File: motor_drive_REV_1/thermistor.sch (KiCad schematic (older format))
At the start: 6 parts, among them J5 Conn_01x02, J6 Conn_01x02

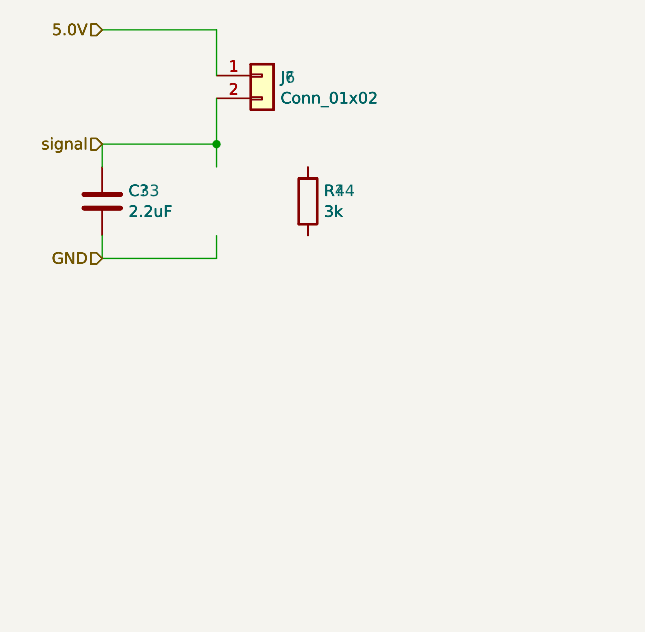
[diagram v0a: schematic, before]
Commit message: started layout
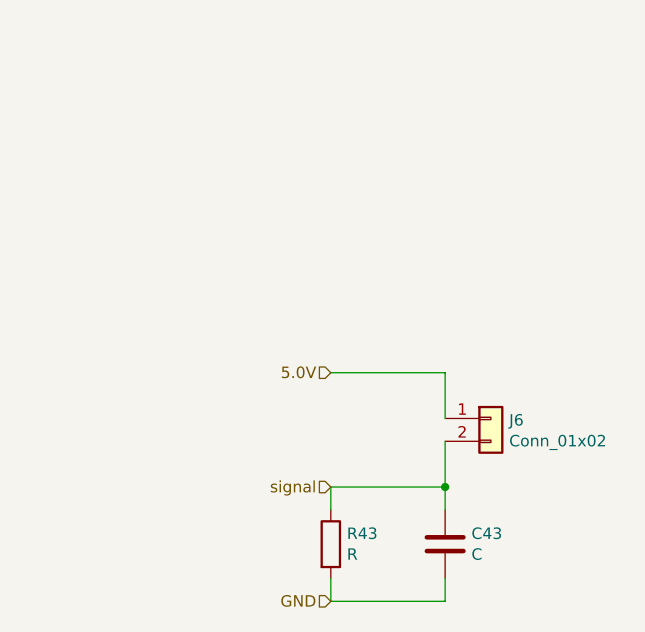
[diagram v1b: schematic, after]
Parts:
- removed C32, C33: 2.2uF, motor_drive_footprints:C_0603_1608Metric, symbol motor_drive:C
- removed J5: Conn_01x02, symbol Connector_Generic:Conn_01x02
- removed R44: 3k, motor_drive_footprints:C_0603_1608Metric, symbol motor_drive:R
- added C43: C, motor_drive_footprints:C_0603_1608Metric, symbol motor_drive:C
- J6: footprint (none) -> motor_drive_footprints:2pos_254
- R43: value 3k -> R
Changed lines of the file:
@@
 $Descr A4 11693 8268
 encoding utf-8
-Sheet 15 15
+Sheet 15 16
 Title ""
 Date ""
@@
 $EndDescr
 $Comp
-L motor_drive:R R44
-U 1 1 5E6227DE
-P 5400 2750
-AR Path="/5E61C379/5E6227DE" Ref="R44"  Part="1"
-AR Path="/5E61FCEC/5E6227DE" Ref="R?"  Part="1"
-AR Path="/5E626DD7/5E6227DE" Ref="R?"  Part="1"
-F 0 "R?" H 5470 2796 50  0000 L CNN
-F 1 "3k" H 5470 2705 50  0000 L CNN
-F 2 "motor_drive_footprints:C_0603_1608Metric" V 5330 2750 50  0001 C CNN
-F 3 "~" H 5400 2750 50  0001 C CNN
-	1    5400 2750
+L motor_drive:R R43
+U 1 1 5E41A8AA
+P 5500 4250
+F 0 "R43" H 5570 4296 50  0000 L CNN
+F 1 "R" H 5570 4205 50  0000 L CNN
+F 2 "motor_drive_footprints:C_0603_1608Metric" V 5430 4250 50  0001 C CNN
+F 3 "~" H 5500 4250 50  0001 C CNN
+	1    5500 4250
 	1    0    0    -1
 $EndComp
 $Comp
-L motor_drive:C C33
-U 1 1 5E6227DF
-P 4500 2750
-AR Path="/5E61C379/5E6227DF" Ref="C33"  Part="1"
-AR Path="/5E61FCEC/5E6227DF" Ref="C?"  Part="1"
-AR Path="/5E626DD7/5E6227DF" Ref="C?"  Part="1"
-F 0 "C?" H 4615 2796 50  0000 L CNN
-F 1 "2.2uF" H 4615 2705 50  0000 L CNN
-F 2 "motor_drive_footprints:C_0603_1608Metric" H 4538 2600 50  0001 C CNN
-F 3 "~" H 4500 2750 50  0001 C CNN
-	1    4500 2750
+L motor_drive:C C43
+U 1 1 5E41AB44
+P 6000 4250
+F 0 "C43" H 6115 4296 50  0000 L CNN
+F 1 "C" H 6115 4205 50  0000 L CNN
+F 2 "motor_drive_footprints:C_0603_1608Metric" H 6038 4100 50  0001 C CNN
+F 3 "~" H 6000 4250 50  0001 C CNN
+	1    6000 4250
 	1    0    0    -1
 $EndComp
 $Comp
 L Connector_Generic:Conn_01x02 J6
-U 1 1 5E6227E0
-P 5200 2200
-AR Path="/5E61C379/5E6227E0" Ref="J6"  Part="1"
-AR Path="/5E61FCEC/5E6227E0" Ref="J?"  Part="1"
-AR Path="/5E626DD7/5E6227E0" Ref="J?"  Part="1"
-F 0 "J?" H 5280 2192 50  0000 L CNN
-F 1 "Conn_01x02" H 5280 2101 50  0000 L CNN
-F 2 "" H 5200 2200 50  0001 C CNN
-F 3 "~" H 5200 2200 50  0001 C CNN
-	1    5200 2200
+U 1 1 5E41B07F
+P 6200 3700
+F 0 "J6" H 6280 3692 50  0000 L CNN
+F 1 "Conn_01x02" H 6280 3601 50  0000 L CNN
+F 2 "motor_drive_footprints:2pos_254" H 6200 3700 50  0001 C CNN
+F 3 "~" H 6200 3700 50  0001 C CNN
+	1    6200 3700
 	1    0    0    -1
 $EndComp
 Wire Wire Line
-	4500 2600 4500 2500
+	5500 3500 6000 3500
 Wire Wire Line
-	4500 2500 5000 2500
+	6000 3500 6000 3700
 Wire Wire Line
-	5000 2500 5000 2600
+	6000 3800 6000 4000
 Wire Wire Line
-	4500 2900 4500 3000
+	5500 4100 5500 4000
 Wire Wire Line
-	4500 3000 5000 3000
+	5500 4000 6000 4000
+Connection ~ 6000 4000
 Wire Wire Line
-	5000 3000 5000 2900
-Text HLabel 4500 3000 0    50   Input ~ 0
+	6000 4000 6000 4100
+Wire Wire Line
+	5500 4400 5500 4500
+Wire Wire Line
+	5500 4500 6000 4500
+Wire Wire Line
+	6000 4500 6000 4400
+Text HLabel 5500 3500 0    50   Input ~ 0
+5.0V
+Text HLabel 5500 4000 0    50   Input ~ 0
+signal
+Text HLabel 5500 4500 0    50   Input ~ 0
 GND
-Text HLabel 4500 2500 0    50   Input ~ 0
-signal
-Text HLabel 4500 2000 0    50   Input ~ 0
-5.0V
-Wire Wire Line
-	4500 2000 5000 2000
-Wire Wire Line
-	5000 2000 5000 2200
-Wire Wire Line
-	5000 2300 5000 2500
-Connection ~ 5000 2500
-$Comp
-L motor_drive:R R?
-U 1 1 5E61C762
-P 5400 2750
-AR Path="/5E61FCEC/5E61C762" Ref="R?"  Part="1"
-AR Path="/5E61C379/5E61C762" Ref="R43"  Part="1"
-AR Path="/5E626DD7/5E61C762" Ref="R?"  Part="1"
-F 0 "R?" H 5470 2796 50  0000 L CNN
-F 1 "3k" H 5470 2705 50  0000 L CNN
-F 2 "motor_drive_footprints:C_0603_1608Metric" V 5330 2750 50  0001 C CNN
-F 3 "~" H 5400 2750 50  0001 C CNN
-	1    5400 2750
-	1    0    0    -1
-$EndComp
-$Comp
-L motor_drive:C C?
-U 1 1 5E61CC30
-P 4500 2750
-AR Path="/5E61FCEC/5E61CC30" Ref="C?"  Part="1"
-AR Path="/5E61C379/5E61CC30" Ref="C32"  Part="1"
-AR Path="/5E626DD7/5E61CC30" Ref="C?"  Part="1"
-F 0 "C?" H 4615 2796 50  0000 L CNN
-F 1 "2.2uF" H 4615 2705 50  0000 L CNN
-F 2 "motor_drive_footprints:C_0603_1608Metric" H 4538 2600 50  0001 C CNN
-F 3 "~" H 4500 2750 50  0001 C CNN
-	1    4500 2750
-	1    0    0    -1
-$EndComp
-$Comp
-L Connector_Generic:Conn_01x02 J?
-U 1 1 5E61D49C
-P 5200 2200
-AR Path="/5E61FCEC/5E61D49C" Ref="J?"  Part="1"
-AR Path="/5E61C379/5E61D49C" Ref="J5"  Part="1"
-AR Path="/5E626DD7/5E61D49C" Ref="J?"  Part="1"
-F 0 "J?" H 5280 2192 50  0000 L CNN
-F 1 "Conn_01x02" H 5280 2101 50  0000 L CNN
-F 2 "" H 5200 2200 50  0001 C CNN
-F 3 "~" H 5200 2200 50  0001 C CNN
-	1    5200 2200
-	1    0    0    -1
-$EndComp
-Text HLabel 4500 3000 0    50   Input ~ 0
-GND
-Text HLabel 4500 2500 0    50   Input ~ 0
-signal
-Text HLabel 4500 2000 0    50   Input ~ 0
-5.0V
 $EndSCHEMATC
